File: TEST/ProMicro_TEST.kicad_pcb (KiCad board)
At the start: 2 copper layers, 17.8 x 30.5 mm, 6 parts

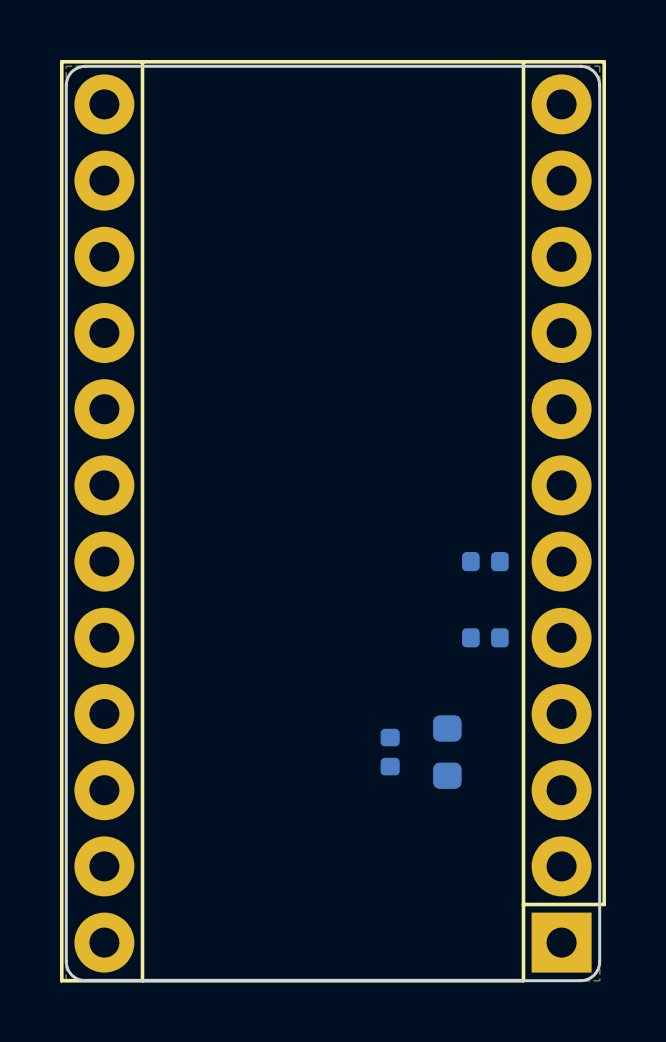
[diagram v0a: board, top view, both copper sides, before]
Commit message: route
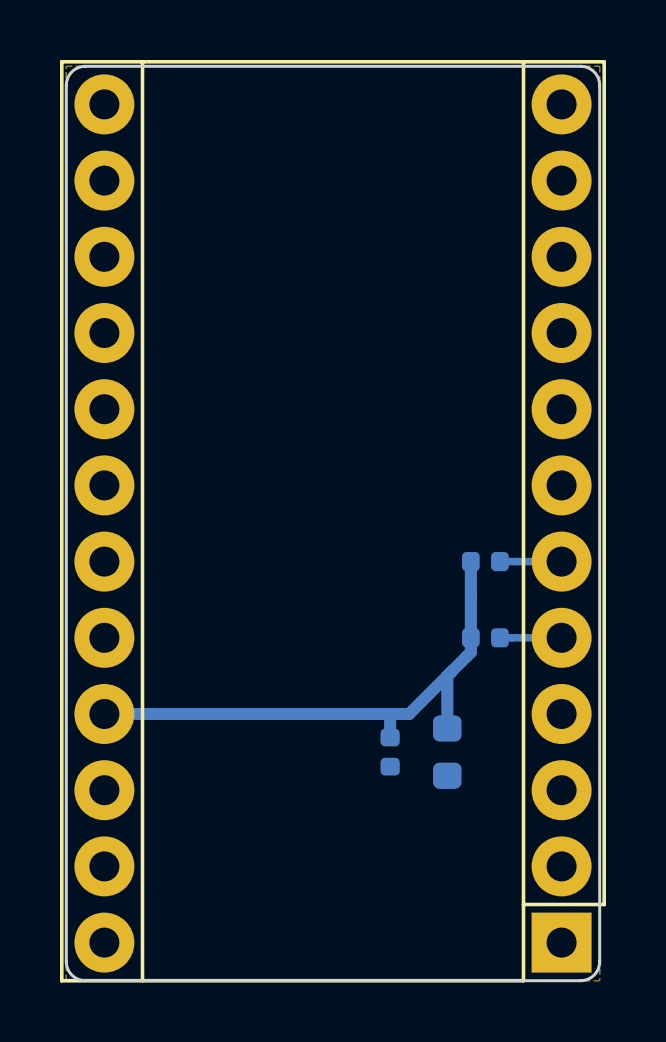
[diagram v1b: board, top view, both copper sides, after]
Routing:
- net +3V3: track 0.00 -> 18.8 mm
- net SDA: track 0.00 -> 2.06 mm
- net SCL: track 0.00 -> 2.03 mm
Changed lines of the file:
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@@
     (thickness 0.8)
     (drawings 67)
-    (tracks 0)
+    (tracks 14)
     (zones 0)
     (modules 6)
@@
     (uvia_dia 0.3)
     (uvia_drill 0.1)
-    (add_net +5V)
-    (add_net BTN)
-    (add_net CIPO)
-    (add_net COPI)
-    (add_net CS0)
-    (add_net CS1)
-    (add_net D8)
-    (add_net INT)
-    (add_net PWM)
-    (add_net RXD)
-    (add_net SCK)
     (add_net SCL)
     (add_net SDA)
-    (add_net STAT)
-    (add_net TCK)
-    (add_net TDI)
-    (add_net TDO)
-    (add_net TMS)
-    (add_net TXD)
-    (add_net ~RST)
   )
   (net_class Power ""
@@
   (gr_line (start 153.035 115.57) (end 136.525 115.57) (layer Edge.Cuts) (width 0.1))
   (gr_line (start 136.525 85.09) (end 153.035 85.09) (layer Edge.Cuts) (width 0.1))
+  (segment (start 146.685 107.465) (end 146.685 106.68) (width 0.4) (layer B.Cu) (net 2))
+  (segment (start 146.685 106.68) (end 147.32 106.68) (width 0.4) (layer B.Cu) (net 2))
+  (segment (start 137.16 106.68) (end 146.685 106.68) (width 0.4) (layer B.Cu) (net 2))
+  (segment (start 148.59 105.41) (end 148.717 105.283) (width 0.4) (layer B.Cu) (net 2))
+  (segment (start 148.59 107.1625) (end 148.59 105.41) (width 0.4) (layer B.Cu) (net 2))
+  (segment (start 147.32 106.68) (end 148.717 105.283) (width 0.4) (layer B.Cu) (net 2))
+  (segment (start 149.225 104.775) (end 148.717 105.283) (width 0.4) (layer B.Cu) (net 2))
+  (segment (start 149.375 104.625) (end 149.225 104.775) (width 0.4) (layer B.Cu) (net 2))
+  (segment (start 149.375 104.14) (end 149.375 104.625) (width 0.4) (layer B.Cu) (net 2))
+  (segment (start 149.375 104.14) (end 149.375 102.72) (width 0.4) (layer B.Cu) (net 2))
+  (segment (start 149.375 101.6) (end 149.375 102.72) (width 0.4) (layer B.Cu) (net 2))
+  (segment (start 152.4 101.6) (end 150.368 101.6) (width 0.25) (layer B.Cu) (net 3))
+  (segment (start 150.345 104.14) (end 150.749 104.14) (width 0.25) (layer B.Cu) (net 4))
+  (segment (start 152.4 104.14) (end 150.749 104.14) (width 0.25) (layer B.Cu) (net 4))
   (zone (net 1) (net_name GND) (layer F.Cu) (hatch edge 0.508)
     (connect_pads (clearance 0.125))
